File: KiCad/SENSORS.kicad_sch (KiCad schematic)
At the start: 8 parts, among them U5 TMP102xxDRL, U6 A1104xLH

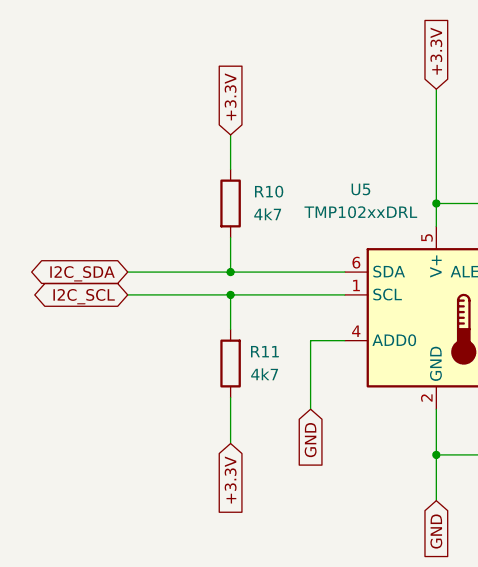
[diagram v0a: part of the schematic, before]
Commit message: Modificacio
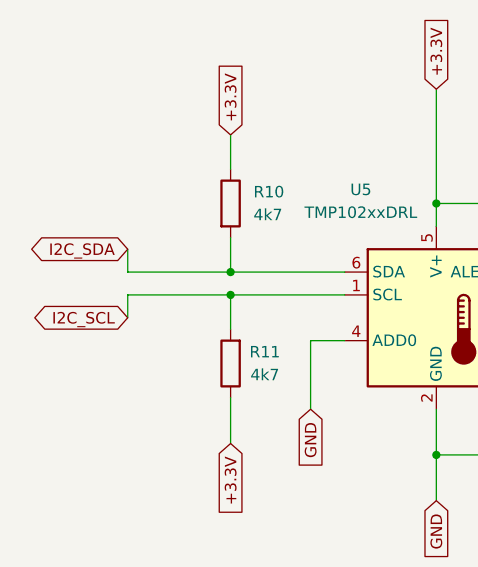
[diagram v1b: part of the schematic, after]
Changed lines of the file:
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@@
+	(wire
+		(pts
+			(xy 66.04 83.82) (xy 66.04 86.36)
+		)
+		(stroke
+			(width 0)
+			(type default)
+		)
+	)
 	(wire
 		(pts
@@
 		(pts
 			(xy 114.3 101.6) (xy 100.33 101.6)
+		)
+		(stroke
+			(width 0)
+			(type default)
+		)
+	)
+	(wire
+		(pts
+			(xy 66.04 78.74) (xy 66.04 81.28)
 		)
 		(stroke
@@
 	(global_label "I2C_SDA"
 		(shape bidirectional)
-		(at 66.04 81.28 180)
-		(fields_autoplaced yes)
-		(effects
-			(font
-				(size 1.27 1.27)
-			)
-			(justify right)
-		)
-		(property "Intersheetrefs" "${INTERSHEET_REFS}"
-			(at 54.3235 81.28 0)
+		(at 66.04 78.74 180)
+		(fields_autoplaced yes)
+		(effects
+			(font
+				(size 1.27 1.27)
+			)
+			(justify right)
+		)
+		(property "Intersheetrefs" "${INTERSHEET_REFS}"
+			(at 54.3235 78.74 0)
 			(effects
 				(font
@@
 	(global_label "I2C_SCL"
 		(shape bidirectional)
-		(at 66.04 83.82 180)
-		(fields_autoplaced yes)
-		(effects
-			(font
-				(size 1.27 1.27)
-			)
-			(justify right)
-		)
-		(property "Intersheetrefs" "${INTERSHEET_REFS}"
-			(at 54.384 83.82 0)
-			(effects
-				(font
+		(at 66.04 86.36 180)
+		(fields_autoplaced yes)
+		(effects
+			(font
+				(size 1.27 1.27)
+			)
+			(justify right)
+		)
+		(property "Intersheetrefs" "${INTERSHEET_REFS}"
+			(at 54.384 86.36 0)
+			(effects
+				(font
